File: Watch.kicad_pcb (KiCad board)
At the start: 2 copper layers, 37 x 39.8 mm, 48 parts, among them J1 USB_C_Receptacle_USB2.0_14P, Q1 2N3904, Q2 2N3904, Q3 2N3904, Q4 2N3904, SW1 SW_Push, SW3 SW_Push, SW4 SW_Push, U1 MCP73831-2-OT, U3 AP2112K-3.3, U7 ATSAMD21E18A-A, Y2 32768Hz

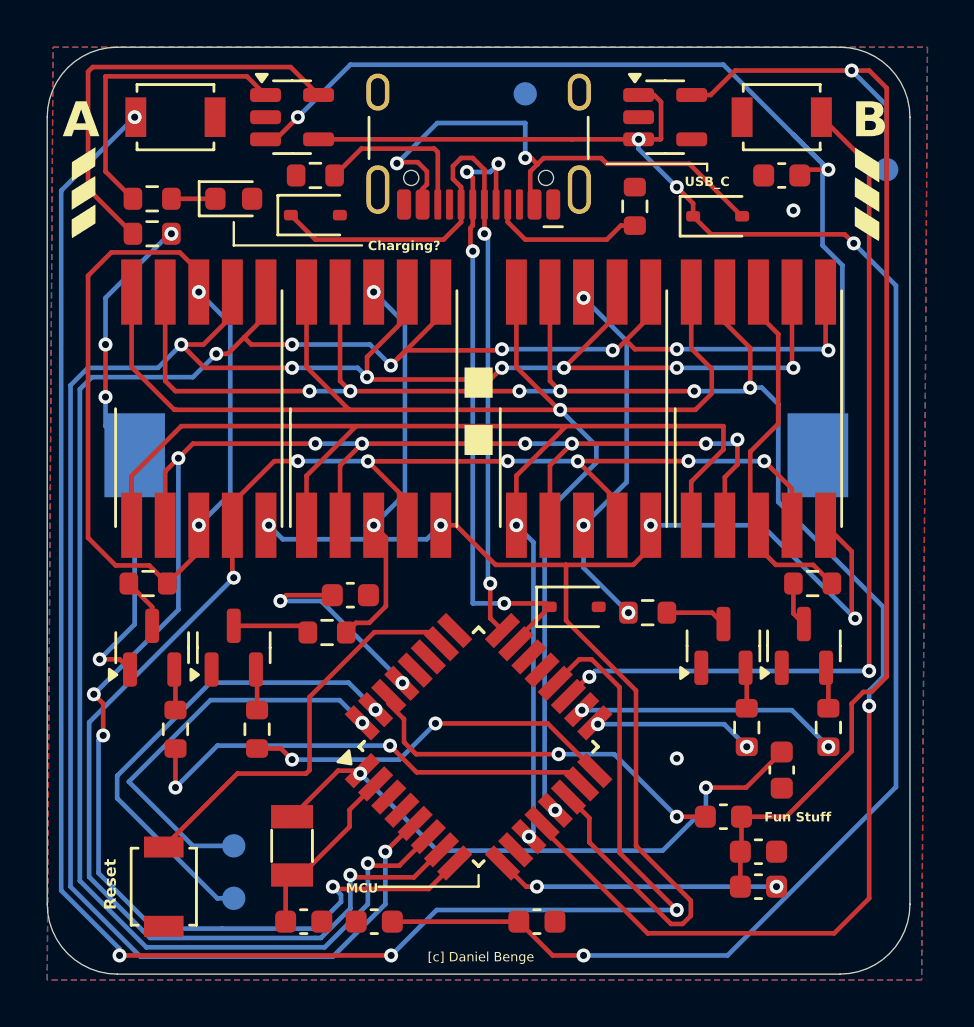
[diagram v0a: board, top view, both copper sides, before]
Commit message: Tiny improvements
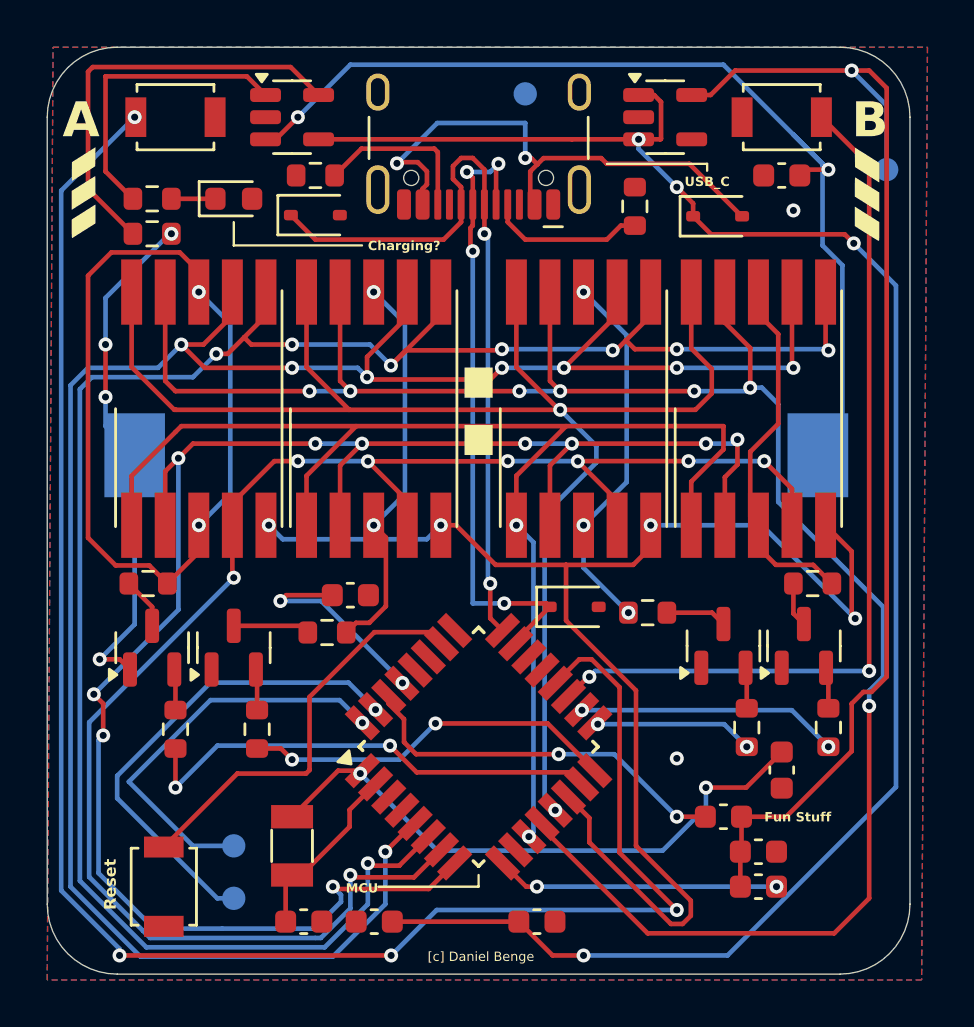
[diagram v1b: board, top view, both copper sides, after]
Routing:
- net G: track 65.4 -> 64.4 mm
